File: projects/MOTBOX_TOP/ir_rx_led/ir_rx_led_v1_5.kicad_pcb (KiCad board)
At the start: 2 copper layers, 23 x 40 mm, 10 parts, among them J1 Conn_01x03

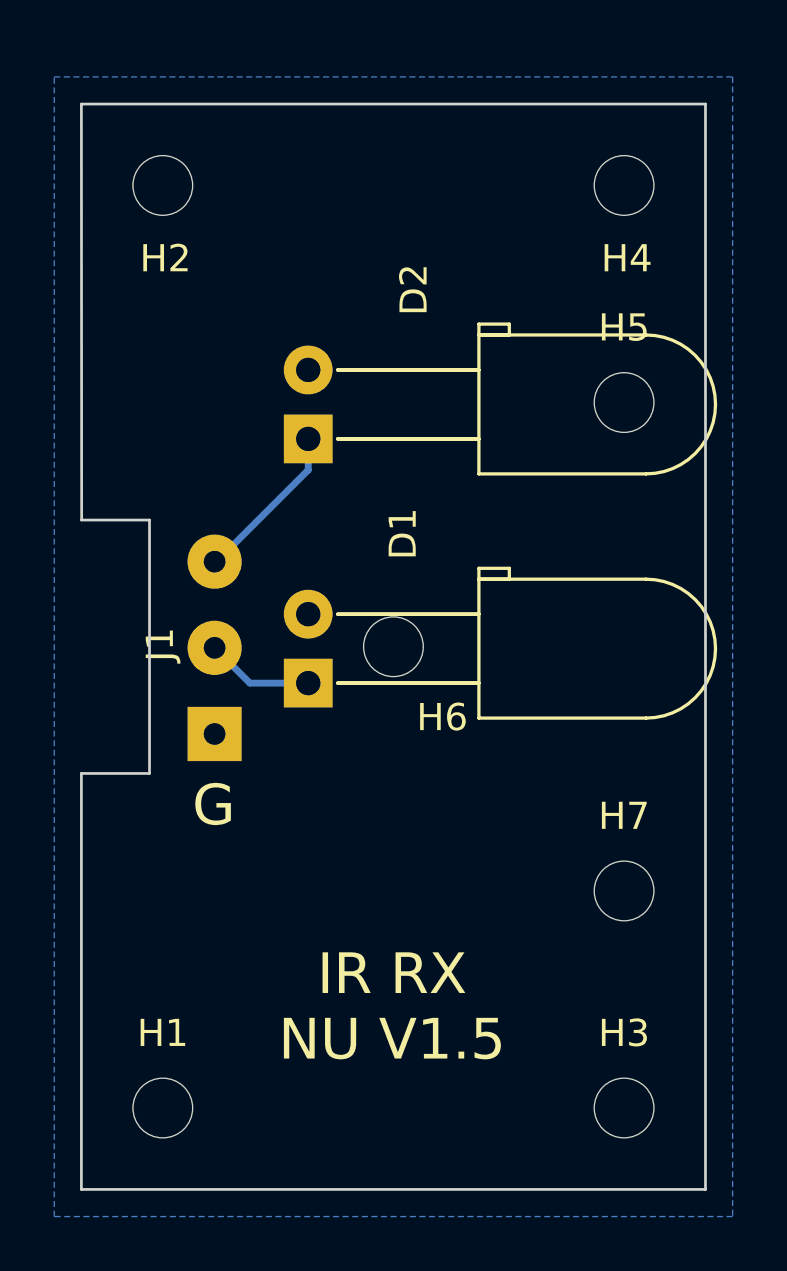
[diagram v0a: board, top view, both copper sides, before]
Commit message: Changes for improvments
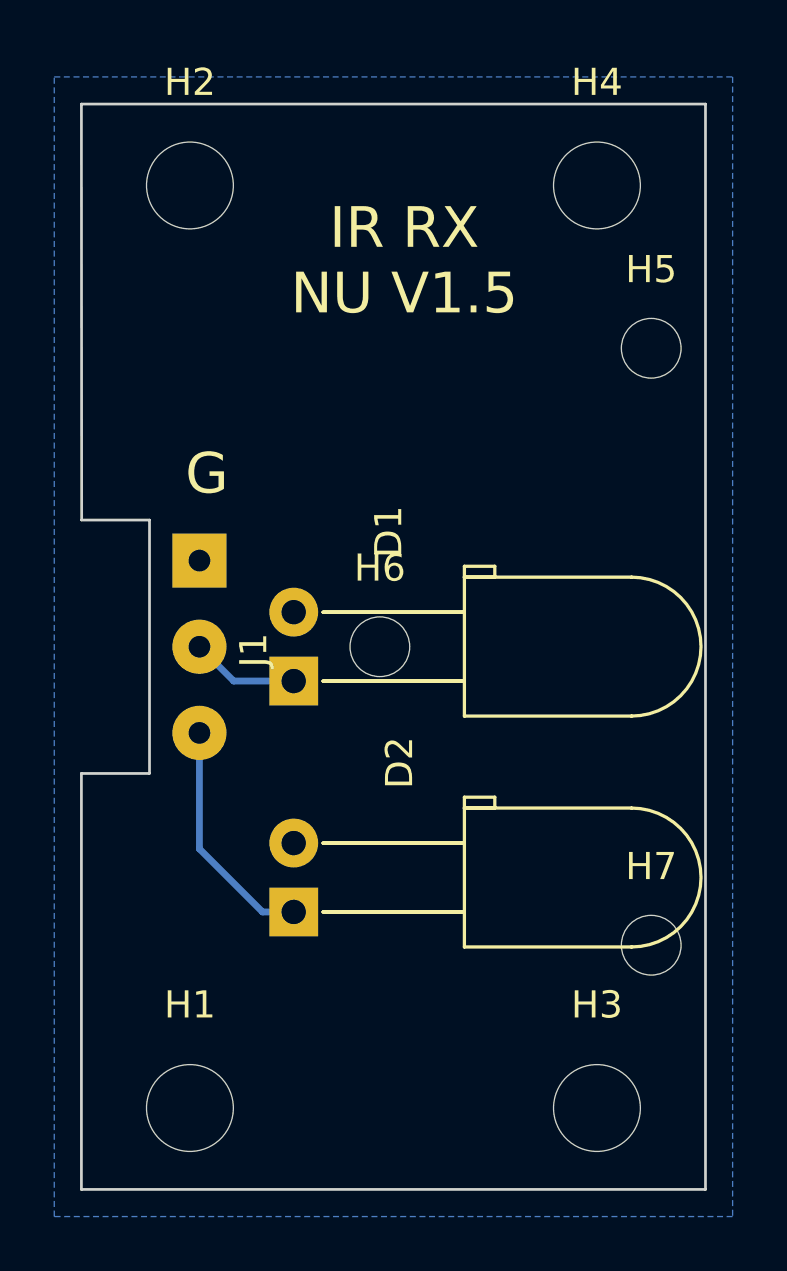
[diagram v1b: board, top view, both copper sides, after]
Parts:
- H1, H2, H3, H4: footprint MountingHole:MountingHole_2.2mm_M2_ISO7380 -> MountingHole:MountingHole_3.2mm_M3_DIN965
- H5, H6, H7: footprint MountingHole:MountingHole_2.2mm_M2_ISO7380 -> MountingHole:MountingHole_2.2mm_M2_DIN965
- moved D2 17.4 mm to (137.8, 60.8)
- moved J1 6.41 mm to (134.3, 47.8), turned to 270 degrees
- moved H5 2.24 mm to (151.0, 40.0)
- moved H7 2.24 mm to (151.0, 62.0)
- moved H1 1.00 mm to (134.0, 68.0)
- moved H2 1.00 mm to (134.0, 34.0)
- moved H3 1.00 mm to (149.0, 68.0)
- moved H4 1.00 mm to (149.0, 34.0)
- moved D1 0.54 mm to (137.8, 52.3)
- moved H6 0.50 mm to (141.0, 51.0)
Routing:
- net Net-(D2-Pad1): track 6.00 -> 8.71 mm
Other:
- board text added: "Hole size and position changes as per the ORG box"
